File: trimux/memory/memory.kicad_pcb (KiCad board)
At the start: 2 copper layers, 23.5 x 45.7 mm, 15 parts, among them U1 trimux, U2 trimux

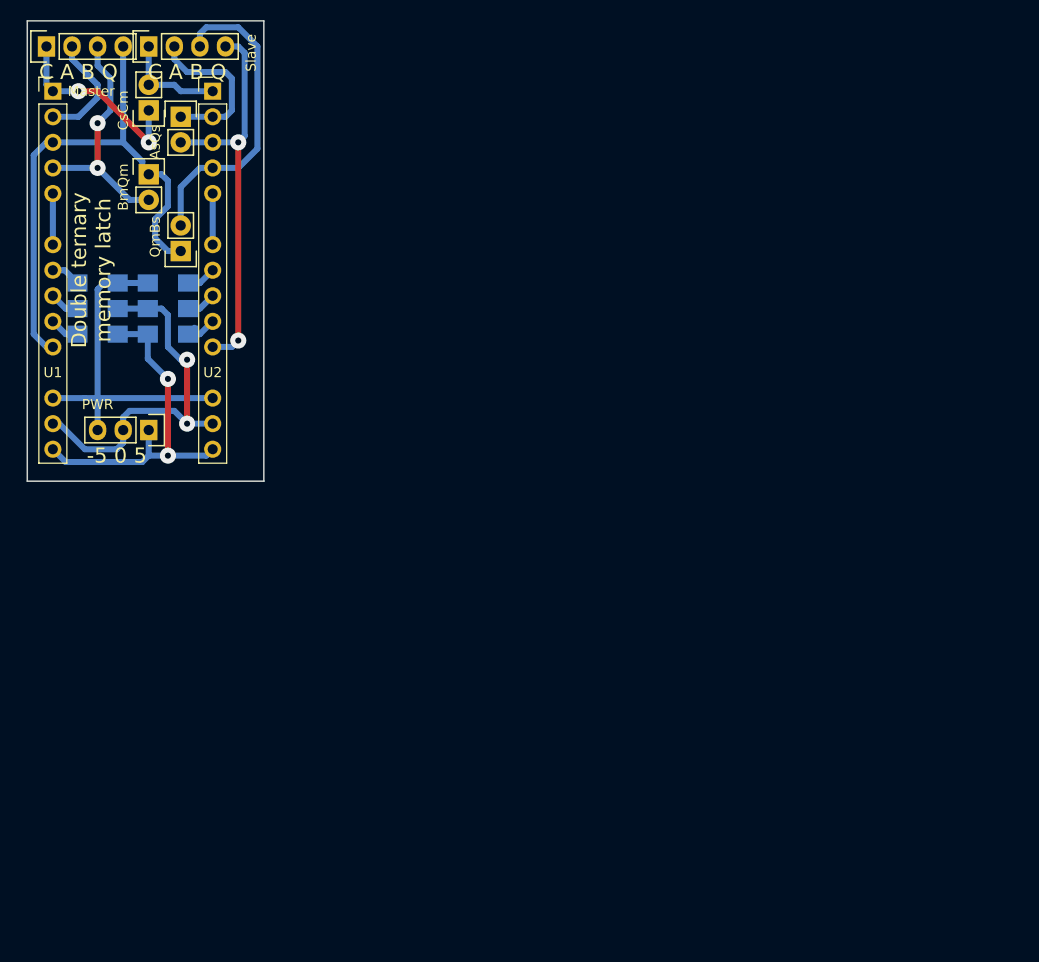
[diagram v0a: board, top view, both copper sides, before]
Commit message: counter board
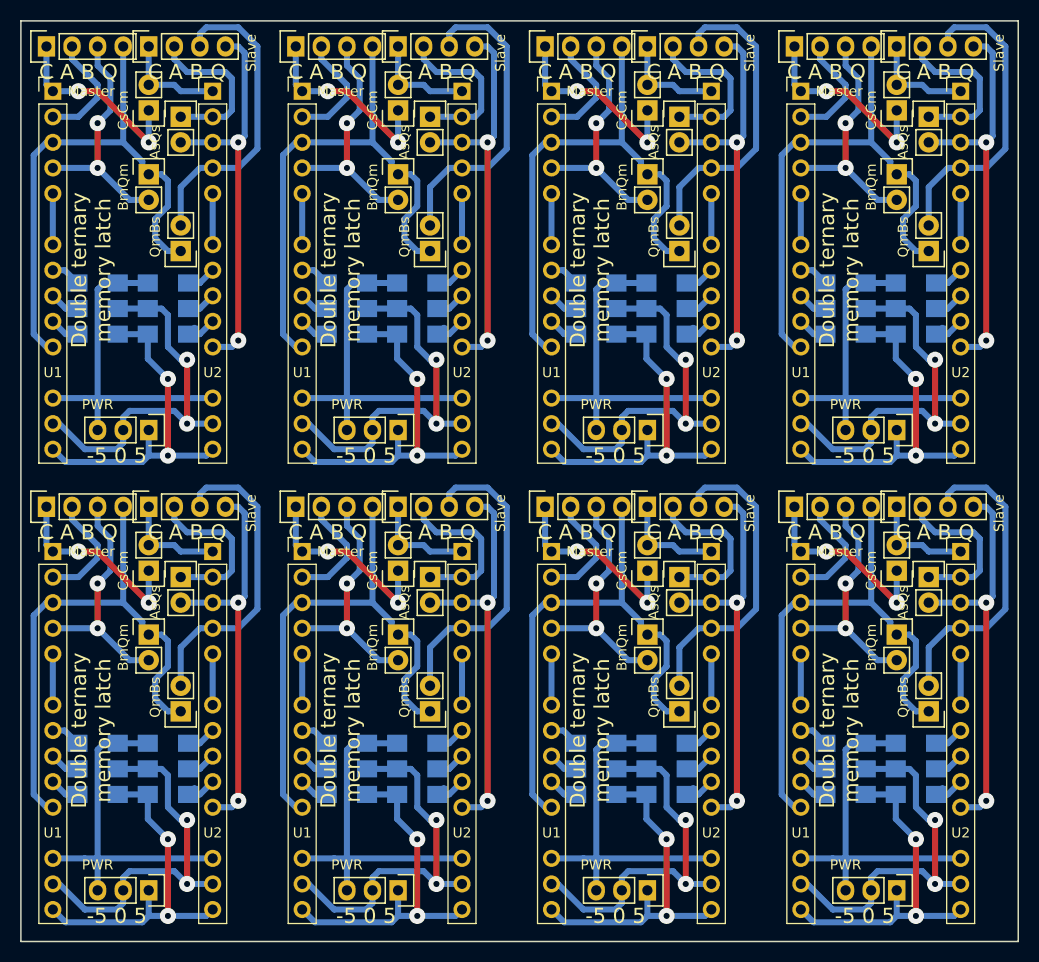
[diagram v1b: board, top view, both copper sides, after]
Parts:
- added AsQs: Jumper_NO_Small, Pin_Headers:Pin_Header_Straight_1x02, F.Cu at (186.1, 85.7)
- added AsQs: Jumper_NO_Small, Pin_Headers:Pin_Header_Straight_1x02, F.Cu at (210.8, 85.7)
- added AsQs: Jumper_NO_Small, Pin_Headers:Pin_Header_Straight_1x02, F.Cu at (260.4, 85.7)
- added AsQs: Jumper_NO_Small, Pin_Headers:Pin_Header_Straight_1x02, F.Cu at (235.6, 85.7)
- added AsQs: Jumper_NO_Small, Pin_Headers:Pin_Header_Straight_1x02, F.Cu at (235.6, 40.0)
- added AsQs: Jumper_NO_Small, Pin_Headers:Pin_Header_Straight_1x02, F.Cu at (260.4, 40.0)
- added AsQs: Jumper_NO_Small, Pin_Headers:Pin_Header_Straight_1x02, F.Cu at (210.8, 40.0)
- added BmQm: Jumper_NO_Small, Pin_Headers:Pin_Header_Straight_1x02, F.Cu at (182.9, 91.4)
- added BmQm: Jumper_NO_Small, Pin_Headers:Pin_Header_Straight_1x02, F.Cu at (207.6, 91.4)
- added BmQm: Jumper_NO_Small, Pin_Headers:Pin_Header_Straight_1x02, F.Cu at (257.2, 91.4)
- added BmQm: Jumper_NO_Small, Pin_Headers:Pin_Header_Straight_1x02, F.Cu at (232.4, 91.4)
- added BmQm: Jumper_NO_Small, Pin_Headers:Pin_Header_Straight_1x02, F.Cu at (232.4, 45.7)
- added BmQm: Jumper_NO_Small, Pin_Headers:Pin_Header_Straight_1x02, F.Cu at (257.2, 45.7)
- added BmQm: Jumper_NO_Small, Pin_Headers:Pin_Header_Straight_1x02, F.Cu at (207.6, 45.7)
- added CsCm: Jumper_NO_Small, Pin_Headers:Pin_Header_Straight_1x02, F.Cu at (182.9, 85.1)
- added CsCm: Jumper_NO_Small, Pin_Headers:Pin_Header_Straight_1x02, F.Cu at (207.6, 85.1)
- added CsCm: Jumper_NO_Small, Pin_Headers:Pin_Header_Straight_1x02, F.Cu at (257.2, 85.1)
- added CsCm: Jumper_NO_Small, Pin_Headers:Pin_Header_Straight_1x02, F.Cu at (232.4, 85.1)
- added CsCm: Jumper_NO_Small, Pin_Headers:Pin_Header_Straight_1x02, F.Cu at (232.4, 39.4)
- added CsCm: Jumper_NO_Small, Pin_Headers:Pin_Header_Straight_1x02, F.Cu at (257.2, 39.4)
- added CsCm: Jumper_NO_Small, Pin_Headers:Pin_Header_Straight_1x02, F.Cu at (207.6, 39.4)
- added Master: CONN_01X04, Pin_Headers:Pin_Header_Straight_1x04, F.Cu at (172.7, 78.7)
- added Master: CONN_01X04, Pin_Headers:Pin_Header_Straight_1x04, F.Cu at (197.5, 78.7)
- added Master: CONN_01X04, Pin_Headers:Pin_Header_Straight_1x04, F.Cu at (247.0, 78.7)
- added Master: CONN_01X04, Pin_Headers:Pin_Header_Straight_1x04, F.Cu at (222.2, 78.7)
- added Master: CONN_01X04, Pin_Headers:Pin_Header_Straight_1x04, F.Cu at (222.2, 33.0)
- added Master: CONN_01X04, Pin_Headers:Pin_Header_Straight_1x04, F.Cu at (247.0, 33.0)
- added Master: CONN_01X04, Pin_Headers:Pin_Header_Straight_1x04, F.Cu at (197.5, 33.0)
- added PWR: CONN_01X03, Pin_Headers:Pin_Header_Straight_1x03, F.Cu at (182.9, 116.8)
- added PWR: CONN_01X03, Pin_Headers:Pin_Header_Straight_1x03, F.Cu at (207.6, 116.8)
- added PWR: CONN_01X03, Pin_Headers:Pin_Header_Straight_1x03, F.Cu at (257.2, 116.8)
- added PWR: CONN_01X03, Pin_Headers:Pin_Header_Straight_1x03, F.Cu at (232.4, 116.8)
- added PWR: CONN_01X03, Pin_Headers:Pin_Header_Straight_1x03, F.Cu at (232.4, 71.1)
- added PWR: CONN_01X03, Pin_Headers:Pin_Header_Straight_1x03, F.Cu at (257.2, 71.1)
- added PWR: CONN_01X03, Pin_Headers:Pin_Header_Straight_1x03, F.Cu at (207.6, 71.1)
- added QmBs: Jumper_NO_Small, Pin_Headers:Pin_Header_Straight_1x02, F.Cu at (186.1, 99.1)
- added QmBs: Jumper_NO_Small, Pin_Headers:Pin_Header_Straight_1x02, F.Cu at (210.8, 99.1)
- added QmBs: Jumper_NO_Small, Pin_Headers:Pin_Header_Straight_1x02, F.Cu at (260.4, 99.1)
- added QmBs: Jumper_NO_Small, Pin_Headers:Pin_Header_Straight_1x02, F.Cu at (235.6, 99.1)
- added QmBs: Jumper_NO_Small, Pin_Headers:Pin_Header_Straight_1x02, F.Cu at (235.6, 53.3)
- added QmBs: Jumper_NO_Small, Pin_Headers:Pin_Header_Straight_1x02, F.Cu at (260.4, 53.3)
- added QmBs: Jumper_NO_Small, Pin_Headers:Pin_Header_Straight_1x02, F.Cu at (210.8, 53.3)
- added R1: 150, Resistors_SMD:R_1206_HandSoldering, B.Cu at (177.8, 102.2)
- added R1: 150, Resistors_SMD:R_1206_HandSoldering, B.Cu at (202.6, 102.2)
- added R1: 150, Resistors_SMD:R_1206_HandSoldering, B.Cu at (252.1, 102.2)
- added R1: 150, Resistors_SMD:R_1206_HandSoldering, B.Cu at (227.3, 102.2)
- added R1: 150, Resistors_SMD:R_1206_HandSoldering, B.Cu at (227.3, 56.5)
- added R1: 150, Resistors_SMD:R_1206_HandSoldering, B.Cu at (252.1, 56.5)
- added R1: 150, Resistors_SMD:R_1206_HandSoldering, B.Cu at (202.6, 56.5)
- added R2: 150, Resistors_SMD:R_1206_HandSoldering, B.Cu at (184.8, 102.2)
- added R2: 150, Resistors_SMD:R_1206_HandSoldering, B.Cu at (209.6, 102.2)
- added R2: 150, Resistors_SMD:R_1206_HandSoldering, B.Cu at (259.1, 102.2)
- added R2: 150, Resistors_SMD:R_1206_HandSoldering, B.Cu at (234.3, 102.2)
- added R2: 150, Resistors_SMD:R_1206_HandSoldering, B.Cu at (234.3, 56.5)
- added R2: 150, Resistors_SMD:R_1206_HandSoldering, B.Cu at (259.1, 56.5)
- added R2: 150, Resistors_SMD:R_1206_HandSoldering, B.Cu at (209.6, 56.5)
- added R3: 150, Resistors_SMD:R_1206_HandSoldering, B.Cu at (177.8, 104.8)
- added R3: 150, Resistors_SMD:R_1206_HandSoldering, B.Cu at (202.6, 104.8)
- added R3: 150, Resistors_SMD:R_1206_HandSoldering, B.Cu at (252.1, 104.8)
- added R3: 150, Resistors_SMD:R_1206_HandSoldering, B.Cu at (227.3, 104.8)
- added R3: 150, Resistors_SMD:R_1206_HandSoldering, B.Cu at (227.3, 59.1)
- added R3: 150, Resistors_SMD:R_1206_HandSoldering, B.Cu at (252.1, 59.1)
- added R3: 150, Resistors_SMD:R_1206_HandSoldering, B.Cu at (202.6, 59.1)
- added R4: 150, Resistors_SMD:R_1206_HandSoldering, B.Cu at (184.8, 104.8)
- added R4: 150, Resistors_SMD:R_1206_HandSoldering, B.Cu at (209.6, 104.8)
- added R4: 150, Resistors_SMD:R_1206_HandSoldering, B.Cu at (259.1, 104.8)
- added R4: 150, Resistors_SMD:R_1206_HandSoldering, B.Cu at (234.3, 104.8)
- added R4: 150, Resistors_SMD:R_1206_HandSoldering, B.Cu at (234.3, 59.1)
- added R4: 150, Resistors_SMD:R_1206_HandSoldering, B.Cu at (259.1, 59.1)
- added R4: 150, Resistors_SMD:R_1206_HandSoldering, B.Cu at (209.6, 59.1)
- added R5: 150, Resistors_SMD:R_1206_HandSoldering, B.Cu at (177.8, 107.3)
- added R5: 150, Resistors_SMD:R_1206_HandSoldering, B.Cu at (202.6, 107.3)
- added R5: 150, Resistors_SMD:R_1206_HandSoldering, B.Cu at (252.1, 107.3)
- added R5: 150, Resistors_SMD:R_1206_HandSoldering, B.Cu at (227.3, 107.3)
- added R5: 150, Resistors_SMD:R_1206_HandSoldering, B.Cu at (227.3, 61.6)
- added R5: 150, Resistors_SMD:R_1206_HandSoldering, B.Cu at (252.1, 61.6)
- added R5: 150, Resistors_SMD:R_1206_HandSoldering, B.Cu at (202.6, 61.6)
- added R6: 150, Resistors_SMD:R_1206_HandSoldering, B.Cu at (184.8, 107.3)
- added R6: 150, Resistors_SMD:R_1206_HandSoldering, B.Cu at (209.6, 107.3)
- added R6: 150, Resistors_SMD:R_1206_HandSoldering, B.Cu at (259.1, 107.3)
- added R6: 150, Resistors_SMD:R_1206_HandSoldering, B.Cu at (234.3, 107.3)
- added R6: 150, Resistors_SMD:R_1206_HandSoldering, B.Cu at (234.3, 61.6)
- added R6: 150, Resistors_SMD:R_1206_HandSoldering, B.Cu at (259.1, 61.6)
- added R6: 150, Resistors_SMD:R_1206_HandSoldering, B.Cu at (209.6, 61.6)
- added Slave: CONN_01X04, Pin_Headers:Pin_Header_Straight_1x04, F.Cu at (182.9, 78.7)
- added Slave: CONN_01X04, Pin_Headers:Pin_Header_Straight_1x04, F.Cu at (207.6, 78.7)
- added Slave: CONN_01X04, Pin_Headers:Pin_Header_Straight_1x04, F.Cu at (257.2, 78.7)
- added Slave: CONN_01X04, Pin_Headers:Pin_Header_Straight_1x04, F.Cu at (232.4, 78.7)
- added Slave: CONN_01X04, Pin_Headers:Pin_Header_Straight_1x04, F.Cu at (232.4, 33.0)
- added Slave: CONN_01X04, Pin_Headers:Pin_Header_Straight_1x04, F.Cu at (257.2, 33.0)
- added Slave: CONN_01X04, Pin_Headers:Pin_Header_Straight_1x04, F.Cu at (207.6, 33.0)
- added U1: trimux, trimux:trimux1x15_2.54, F.Cu at (173.4, 83.2)
- added U1: trimux, trimux:trimux1x15_2.54, F.Cu at (198.1, 83.2)
- added U1: trimux, trimux:trimux1x15_2.54, F.Cu at (247.7, 83.2)
- added U1: trimux, trimux:trimux1x15_2.54, F.Cu at (222.9, 83.2)
- added U1: trimux, trimux:trimux1x15_2.54, F.Cu at (222.9, 37.5)
- added U1: trimux, trimux:trimux1x15_2.54, F.Cu at (247.7, 37.5)
- added U1: trimux, trimux:trimux1x15_2.54, F.Cu at (198.1, 37.5)
- added U2: trimux, trimux:trimux1x15_2.54, F.Cu at (189.2, 83.2)
- added U2: trimux, trimux:trimux1x15_2.54, F.Cu at (214.0, 83.2)
- added U2: trimux, trimux:trimux1x15_2.54, F.Cu at (263.5, 83.2)
- added U2: trimux, trimux:trimux1x15_2.54, F.Cu at (238.8, 83.2)
- added U2: trimux, trimux:trimux1x15_2.54, F.Cu at (238.8, 37.5)
- added U2: trimux, trimux:trimux1x15_2.54, F.Cu at (263.5, 37.5)
- added U2: trimux, trimux:trimux1x15_2.54, F.Cu at (214.0, 37.5)
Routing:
- net /Qm: track 54.9 -> 438.8 mm
- net /Qs: track 40.8 -> 326.4 mm, vias 2 -> 16
- net GNDREF: track 37.7 -> 301.8 mm, vias 2 -> 16
- net +5V: track 35.3 -> 282.8 mm, vias 2 -> 16
- net -5V: track 35.1 -> 280.7 mm
- net /Bs: track 31.2 -> 249.6 mm
- net /Bm: track 24.0 -> 191.7 mm, vias 2 -> 16
- net /Cm: track 20.1 -> 161.2 mm, vias 2 -> 16
- net /As: track 16.3 -> 130.3 mm
- net /Am: track 12.0 -> 96.0 mm
- net /Cs: track 10.4 -> 83.4 mm
- net Net-(U2-Pad5): track 5.08 -> 40.6 mm
- net Net-(U1-Pad5): track 5.08 -> 40.6 mm
- net Net-(R6-Pad1): track 3.87 -> 31.0 mm
- net Net-(R3-Pad1): track 2.97 -> 23.8 mm
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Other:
- board size 23.5 x 45.7 mm -> 99.1 x 91.4 mm
